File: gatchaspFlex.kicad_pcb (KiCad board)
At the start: 2 copper layers, 46.6 x 90.3 mm, 22 parts

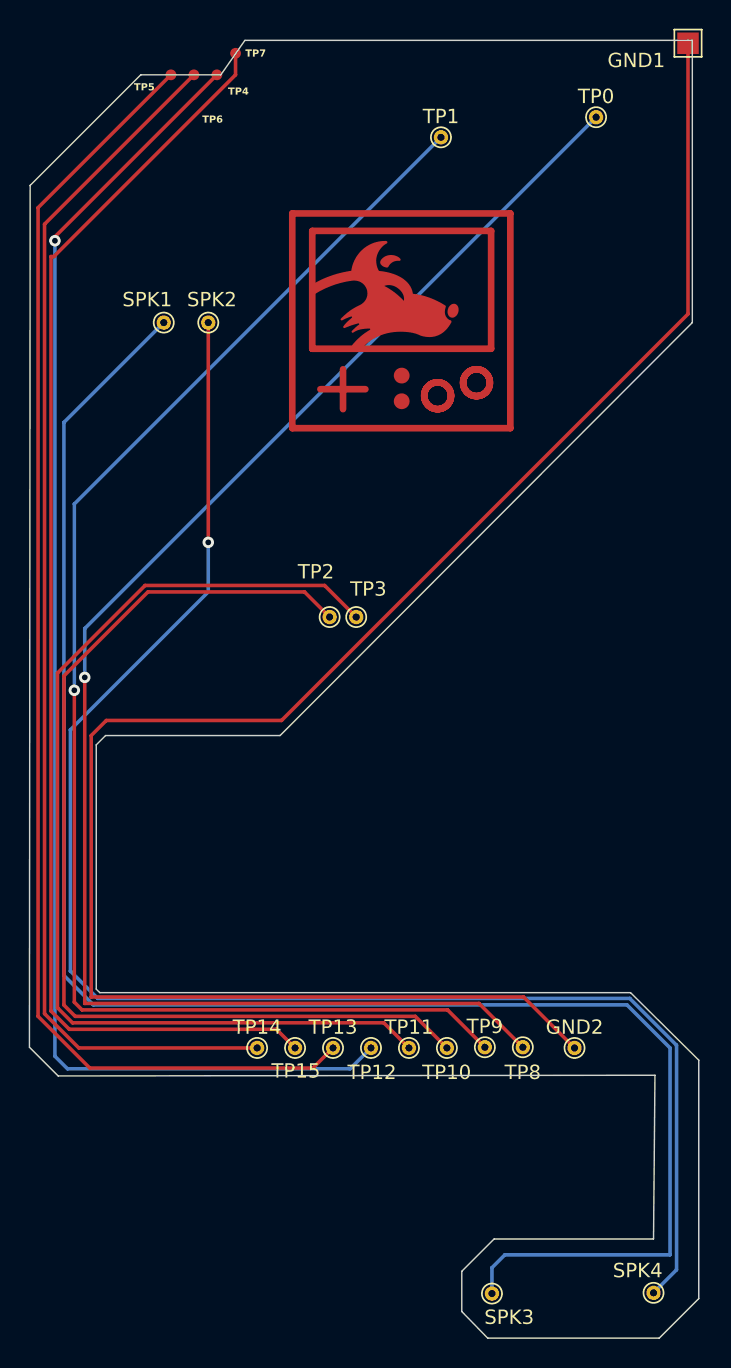
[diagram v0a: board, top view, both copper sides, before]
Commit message: Add files via upload
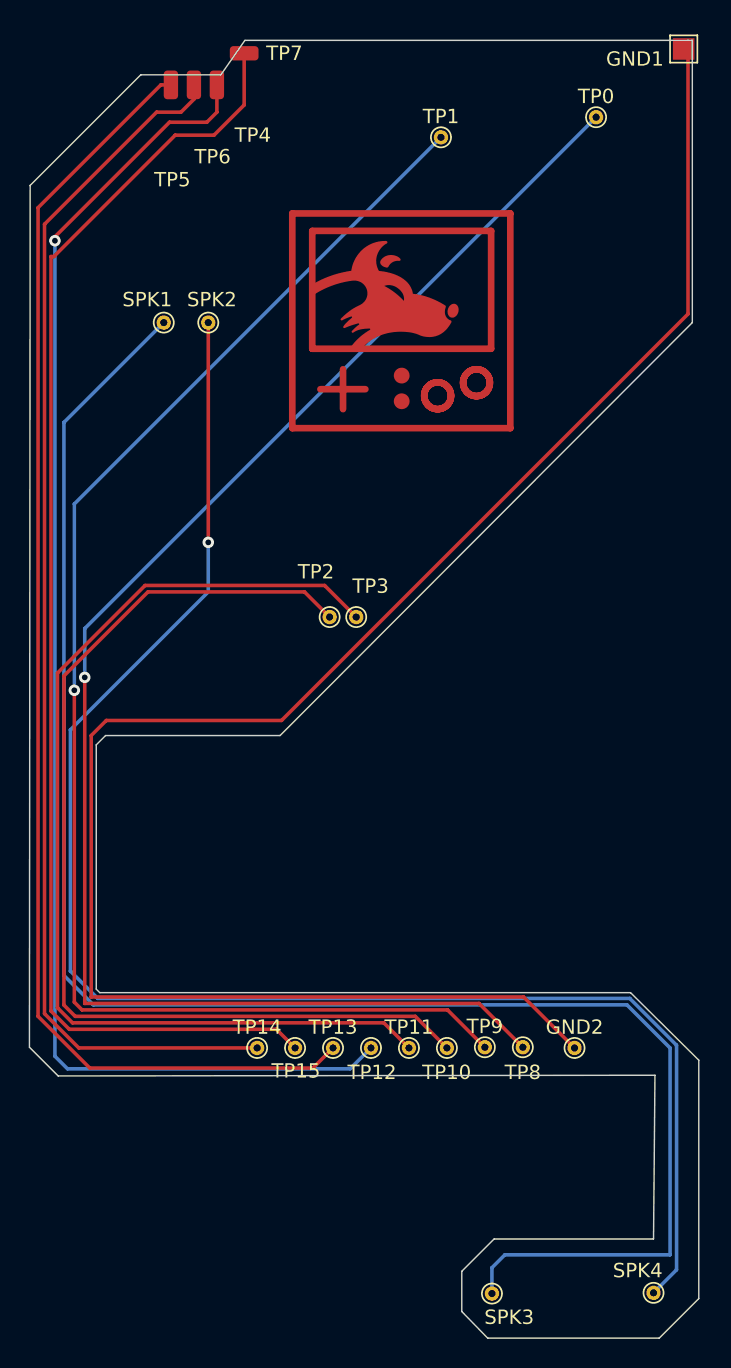
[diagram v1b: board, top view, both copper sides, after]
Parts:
- TP4, TP5, TP6, TP7: footprint SparkFun-Connector:TestPoint-0.75mm -> Connector_Wire:SolderWirePad_1x01_SMD_1x2mm
- moved TP4 0.70 mm to (182.7, 65.0)
- moved TP5 0.70 mm to (179.5, 65.0)
- moved TP6 0.70 mm to (181.1, 65.0)
- moved TP7 0.60 mm to (184.6, 62.8), turned to -90 degrees
- moved GND1 0.50 mm to (215.2, 62.5)
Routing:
- net Net-(TP15-Pad1): track 90.2 -> 92.0 mm
- net Net-(TP12-Pad1): track 96.4 -> 97.2 mm
